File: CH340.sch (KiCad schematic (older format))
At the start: 13 parts, among them J5 USB_B_Micro, J7 Conn_01x04_Female_UART, U5 CH340C

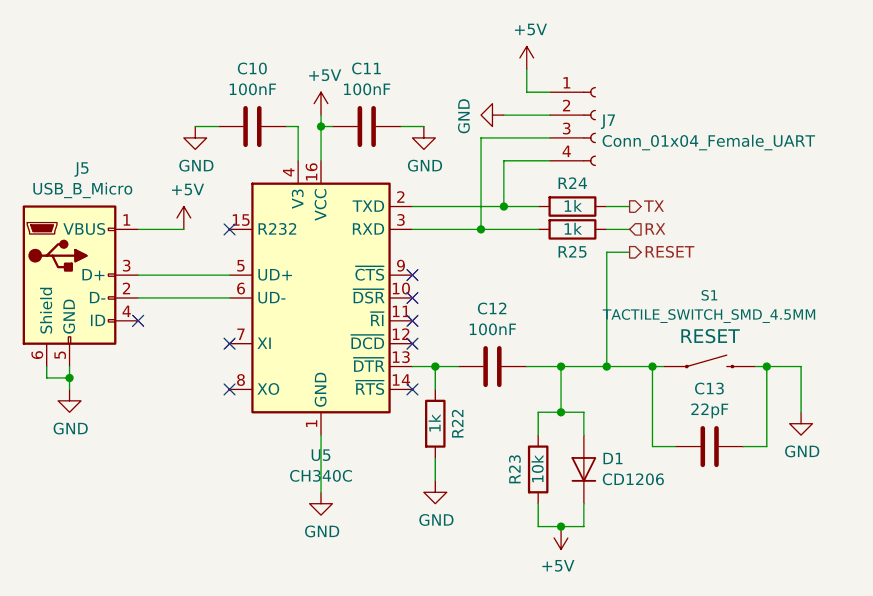
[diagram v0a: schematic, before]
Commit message: DEL-CH340C-UNNEC
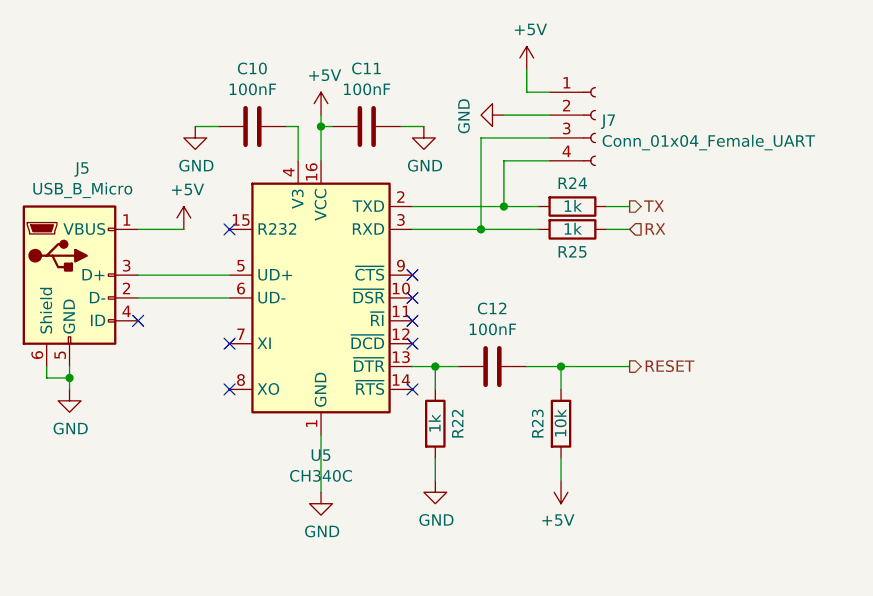
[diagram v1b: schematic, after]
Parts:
- removed C13: 22pF, Capacitor_SMD:C_0603_1608Metric_Pad1.05x0.95mm_HandSolder, symbol Device:C
- removed D1: CD1206, Diode_SMD:D_1206_3216Metric_Pad1.42x1.75mm_HandSolder, symbol Device:D
- removed S1: TACTILE_SWITCH_SMD_4.5MM, Switches:TACTILE_SWITCH_SMD_4.5MM, symbol SparkFun-Switches:MOMENTARY-SWITCH-SPST-SMD-4.5MM
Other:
- moved on the sheet: R23
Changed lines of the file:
@@
 	4650 2950 4650 3050
-$Comp
-L SparkFun-Switches:MOMENTARY-SWITCH-SPST-SMD-4.5MM S1
-U 1 1 5E63B4DB
-P 5850 2550
-F 0 "S1" H 5850 2860 45  0000 C CNN
-F 1 "TACTILE_SWITCH_SMD_4.5MM" H 5850 2776 45  0000 C CNN
-F 2 "Switches:TACTILE_SWITCH_SMD_4.5MM" H 5850 2750 20  0001 C CNN
-F 3 "" H 5850 2550 50  0001 C CNN
-F 4 "RESET" H 5850 2681 60  0000 C CNN "Field4"
-	1    5850 2550
-	1    0    0    -1
-$EndComp
-$Comp
-L Device:C C13
-U 1 1 5E63DB8E
-P 5850 2900
-F 0 "C13" V 5598 2900 50  0000 C CNN
-F 1 "22pF" V 5689 2900 50  0000 C CNN
-F 2 "Capacitor_SMD:C_0603_1608Metric_Pad1.05x0.95mm_HandSolder" H 5888 2750 50  0001 C CNN
-F 3 "~" H 5850 2900 50  0001 C CNN
-	1    5850 2900
-	0    1    1    0
-$EndComp
 $Comp
 L Device:R R23
 U 1 1 5E63EFA7
-P 5100 3000
-F 0 "R23" V 5000 3000 50  0000 C CNN
-F 1 "10k" V 5100 3000 50  0000 C CNN
-F 2 "Resistor_SMD:R_0603_1608Metric_Pad1.05x0.95mm_HandSolder" V 5030 3000 50  0001 C CNN
-F 3 "~" H 5100 3000 50  0001 C CNN
-	1    5100 3000
+P 5200 2800
+F 0 "R23" V 5100 2800 50  0000 C CNN
+F 1 "10k" V 5200 2800 50  0000 C CNN
+F 2 "Resistor_SMD:R_0603_1608Metric_Pad1.05x0.95mm_HandSolder" V 5130 2800 50  0001 C CNN
+F 3 "~" H 5200 2800 50  0001 C CNN
+	1    5200 2800
 	1    0    0    -1
-$EndComp
-$Comp
-L Device:D D1
-U 1 1 5E64106C
-P 5300 3000
-F 0 "D1" V 5346 2921 50  0000 R CNN
-F 1 "CD1206" V 5255 2921 50  0000 R CNN
-F 2 "Diode_SMD:D_1206_3216Metric_Pad1.42x1.75mm_HandSolder" H 5300 3000 50  0001 C CNN
-F 3 "~" H 5300 3000 50  0001 C CNN
-	1    5300 3000
-	0    -1   -1   0
 $EndComp
 $Comp
 L power:+5V #PWR0156
 U 1 1 5E642C88
-P 5200 3250
-F 0 "#PWR0156" H 5200 3100 50  0001 C CNN
-F 1 "+5V" H 5215 3423 50  0000 C CNN
-F 2 "" H 5200 3250 50  0001 C CNN
-F 3 "" H 5200 3250 50  0001 C CNN
-	1    5200 3250
+P 5200 3050
+F 0 "#PWR0156" H 5200 2900 50  0001 C CNN
+F 1 "+5V" H 5215 3223 50  0000 C CNN
+F 2 "" H 5200 3050 50  0001 C CNN
+F 3 "" H 5200 3050 50  0001 C CNN
+	1    5200 3050
 	-1   0    0    1
 $EndComp
-$Comp
-L power:GND #PWR0157
-U 1 1 5E6441EA
-P 6250 2750
-F 0 "#PWR0157" H 6250 2500 50  0001 C CNN
-F 1 "GND" H 6255 2577 50  0000 C CNN
-F 2 "" H 6250 2750 50  0001 C CNN
-F 3 "" H 6250 2750 50  0001 C CNN
-	1    6250 2750
-	1    0    0    -1
-$EndComp
-Wire Wire Line
-	6050 2550 6100 2550
-Wire Wire Line
-	6250 2550 6250 2750
-Wire Wire Line
-	6000 2900 6100 2900
-Wire Wire Line
-	6100 2900 6100 2550
-Connection ~ 6100 2550
-Wire Wire Line
-	6100 2550 6250 2550
-Wire Wire Line
-	5600 2900 5600 2550
-Wire Wire Line
-	5600 2900 5700 2900
-Connection ~ 5600 2550
-Wire Wire Line
-	5600 2550 5650 2550
-Wire Wire Line
-	5100 3150 5100 3250
-Wire Wire Line
-	5100 3250 5200 3250
-Wire Wire Line
-	5300 3150 5300 3250
-Wire Wire Line
-	5300 3250 5200 3250
-Connection ~ 5200 3250
-Text HLabel 5500 2050 2    50   Output ~ 0
+Text HLabel 5500 2550 2    50   Output ~ 0
 RESET
 Wire Wire Line
@@
 Wire Wire Line
 	4550 1950 4850 1950
-Wire Wire Line
-	5500 2050 5400 2050
-Wire Wire Line
-	5400 2050 5400 2550
-Connection ~ 5400 2550
-Wire Wire Line
-	5400 2550 5600 2550
-Wire Wire Line
-	5100 2850 5100 2750
-Wire Wire Line
-	5100 2750 5200 2750
-Wire Wire Line
-	5300 2750 5300 2850
-Connection ~ 5200 2750
-Wire Wire Line
-	5200 2750 5300 2750
-Wire Wire Line
-	5050 2550 5200 2550
-Wire Wire Line
-	5200 2550 5200 2750
-Connection ~ 5200 2550
-Wire Wire Line
-	5200 2550 5400 2550
 Wire Wire Line
 	3350 2150 3750 2150
@@
 Wire Wire Line
 	3350 1950 3550 1950
+Wire Wire Line
+	5050 2550 5200 2550
+Wire Wire Line
+	5200 2650 5200 2550
+Connection ~ 5200 2550
+Wire Wire Line
+	5200 2550 5500 2550
+Wire Wire Line
+	5200 2950 5200 3050
 $EndSCHEMATC
